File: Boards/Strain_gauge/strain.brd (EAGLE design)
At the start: 160 x 100 mm, 69 parts, among them U1 ADS1262IPW, U2 STM32F103CBT6

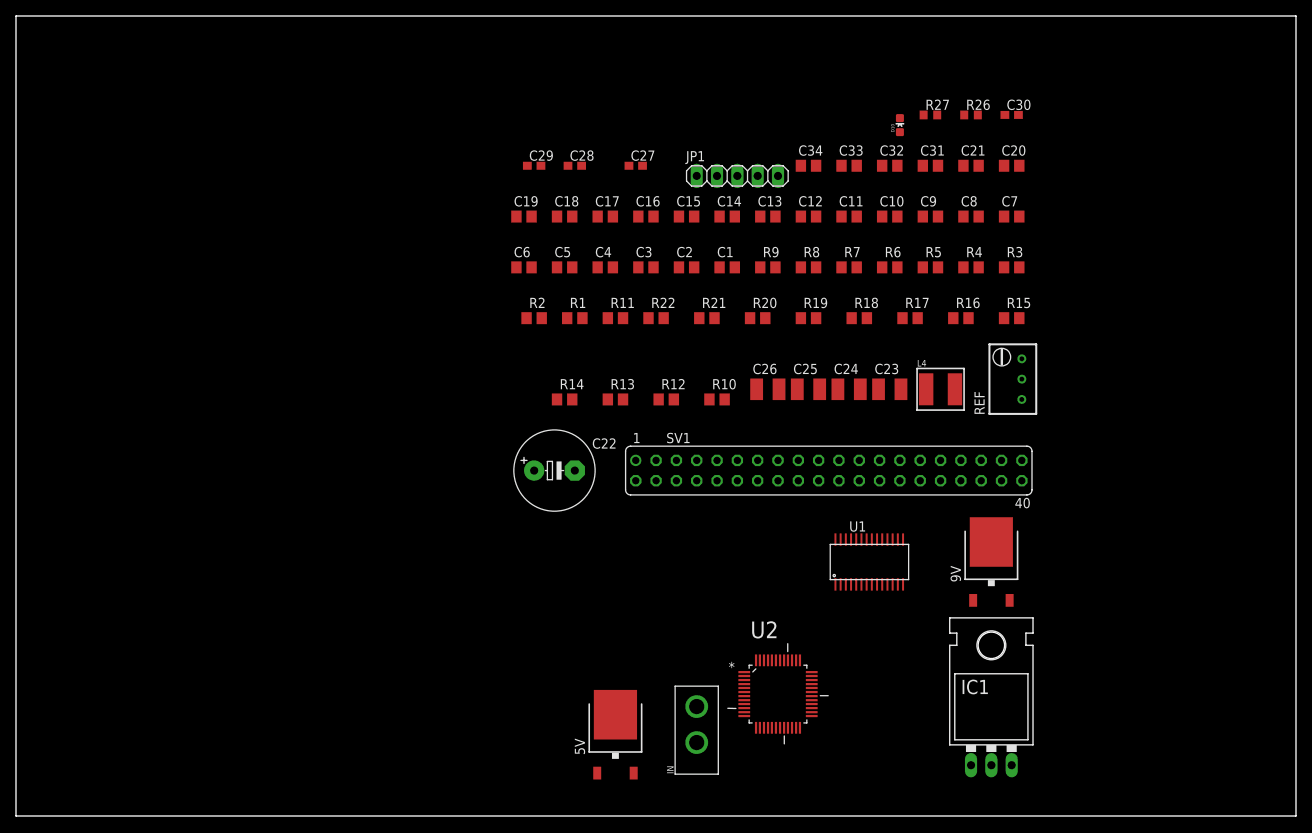
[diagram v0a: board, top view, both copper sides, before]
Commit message: Rushed the fuck out of the ADS1262 board, but here it is
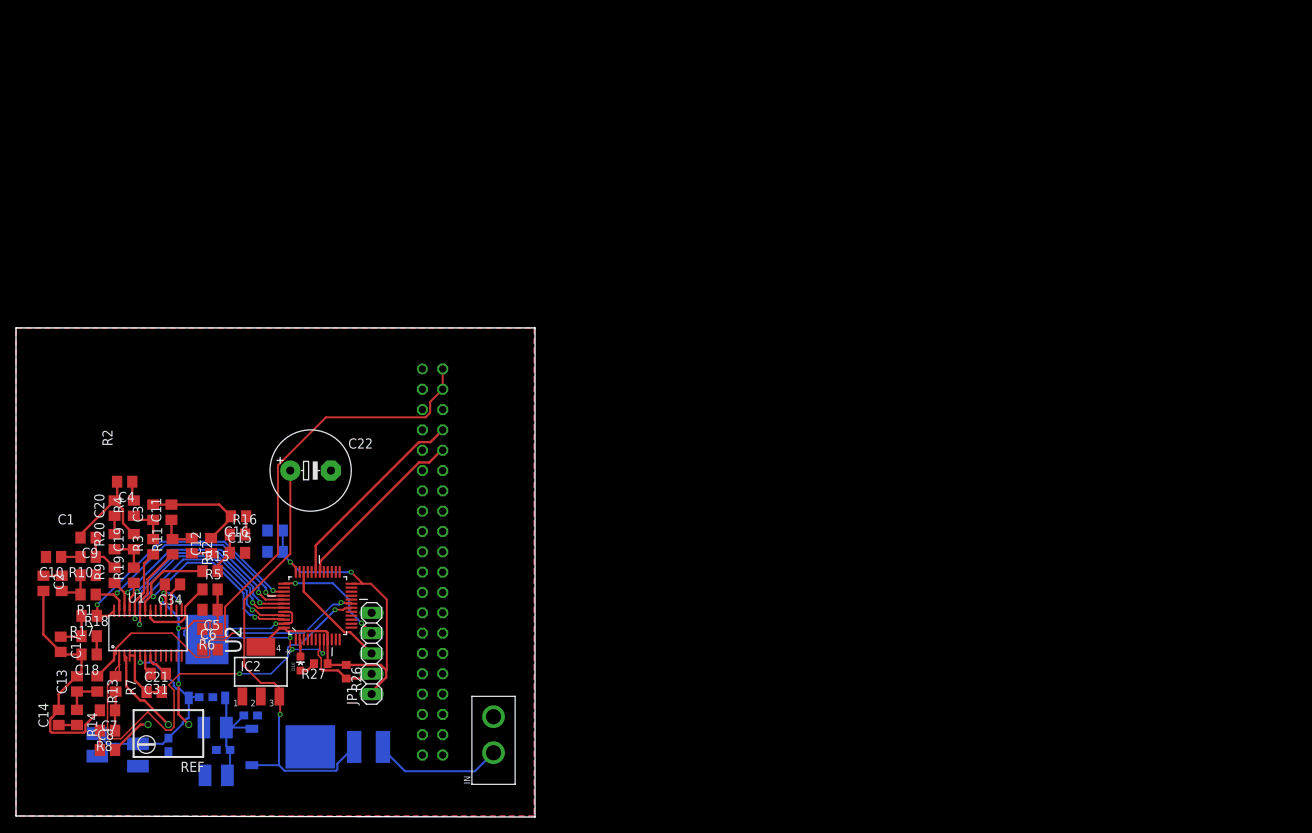
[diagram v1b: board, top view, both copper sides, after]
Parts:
- removed IC1: (no value), v-reg-3:317TL
- removed R21, R22: 750, rcl:R0805
- added IC2: 317EMP, linear:SOT223
- moved C30 131.6 mm to (19.1, 8.89), flipped to the bottom, turned to 270 degrees
- moved C7 128.8 mm to (11.4, 13.2), turned to 180 degrees
- moved C8 126.9 mm to (11.4, 8.26)
- moved C21 121.5 mm to (17.3, 15.5)
- moved C20 120.0 mm to (12.3, 38.5), turned to 90 degrees
- moved C31 115.5 mm to (17.8, 17.8), turned to 180 degrees
- moved REF 114.4 mm to (19.1, 10.2), turned to 90 degrees
- moved R3 112.9 mm to (17.1, 33.7), turned to 90 degrees
- moved C10 112.8 mm to (4.70, 32.4), turned to 180 degrees
- moved C9 112.7 mm to (9.02, 34.8), turned to 180 degrees
- moved R17 109.2 mm to (9.14, 25.0), turned to 180 degrees
- moved R4 108.9 mm to (14.7, 38.5), turned to 90 degrees
- moved R7 105.4 mm to (12.4, 16.5), turned to 270 degrees
- moved R15 105.1 mm to (24.3, 30.6)
- moved R8 105.0 mm to (11.4, 10.7), turned to 180 degrees
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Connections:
- net CAN_RX renamed PA11
- removed net APPS_EN: U2.40
- removed net BRAKE_LIGHT_EN: U2.26
- removed net BRAKE_PRESSURE_F_3_3: U2.10
- removed net BTSF_EN: U2.41
- removed net CAN_STBY: U2.31
- removed net CAN_TX: U2.33
- removed net FAULT_BMS_STATUS_3_3: U2.12
- removed net FAULT_BSPD_STATUS_3_3: U2.27
- removed net FAULT_IMD_STATUS_3_3: U2.13
- removed net HV_CONNECTED_3_3: U2.21
- removed net N$27: IC1.1, R21.1, R22.1
- removed net PRECHARGE_COMPLETE_3_3: U2.42
- removed net RTDS_EN: U2.39
- removed net RTD_EN: U2.45
- removed net SPI1_MISO: U2.16
- removed net SPI1_MOSI: U2.17
- removed net SPI1_NSS: U2.14
- removed net SPI1_SCK: U2.15
- removed net THROTTLE_A_F_3_3: U2.18
- removed net THROTTLE_B_F_3_3: U2.19
- removed net TSAL_HV_EN: U2.22
- removed net TSAL_LV_EN: U2.25
- new net RX: SV1.10, U2.30
- new net TX: SV1.8, U2.31
- net +3V3: now also IC2.4; no longer IC1.2, R21.2, SV1.1, SV1.17
- net ADC_0: now also U2.18
- net ADC_1: now also U2.19
- net ADC_2: now also U2.39
- net ADC_3: now also U2.40
- net ADC_4: now also U2.41
- net ADC_5: now also U2.42
- net ADC_6: now also U2.43
- net ADC_7: now also U2.45
- net ADC_8: now also U2.46
- net CS: no longer SV1.13
- net DIN: no longer SV1.16
- net DOUT: no longer SV1.18
- net DRDY: no longer SV1.22
- net GND: now also IC2.1; no longer R22.2, SV1.14, SV1.20, SV1.25, SV1.30, SV1.34, SV1.39, SV1.9
- net IN_F: now also IC2.3; no longer IC1.3
- net RESET: no longer SV1.36
- net SCLK: no longer SV1.15
- net START: no longer SV1.11
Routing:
- net GND: track 0.00 -> 101.5 mm, vias 0 -> 4
- net 5V: track 0.00 -> 78.6 mm, vias 0 -> 3
- net ADC_0: track 0.00 -> 58.1 mm, vias 0 -> 2
- net IN_F: track 0.00 -> 57.0 mm, vias 0 -> 1
- net +3V3: track 0.00 -> 55.2 mm, vias 0 -> 2
- net ADC_1: track 0.00 -> 40.0 mm, vias 0 -> 2
- net ADC_7: track 0.00 -> 37.4 mm, vias 0 -> 2
- net ADC_6: track 0.00 -> 35.9 mm, vias 0 -> 2
- net ADC_8: track 0.00 -> 33.6 mm, vias 0 -> 2
- net ADC_2: track 0.00 -> 33.0 mm, vias 0 -> 2
- net ADC_3: track 0.00 -> 31.4 mm, vias 0 -> 2
- net ADC_4: track 0.00 -> 29.2 mm, vias 0 -> 2
- net ADC_5: track 0.00 -> 27.9 mm, vias 0 -> 2
- net ANALOG5V: track 0.00 -> 26.3 mm, vias 0 -> 1
- net TX: track 0.00 -> 25.2 mm
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- added copper zone on layer 1, net GND
- added copper zone on layer 16, net GND
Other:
- board size 160 x 100 mm -> 64.9 x 61.1 mm
- board text added: "IFE 2018 ADS1262 BOARD HARRIS MOHAMED"
